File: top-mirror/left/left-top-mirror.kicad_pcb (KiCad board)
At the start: 2 copper layers, 137.8 x 95 mm, 30 parts

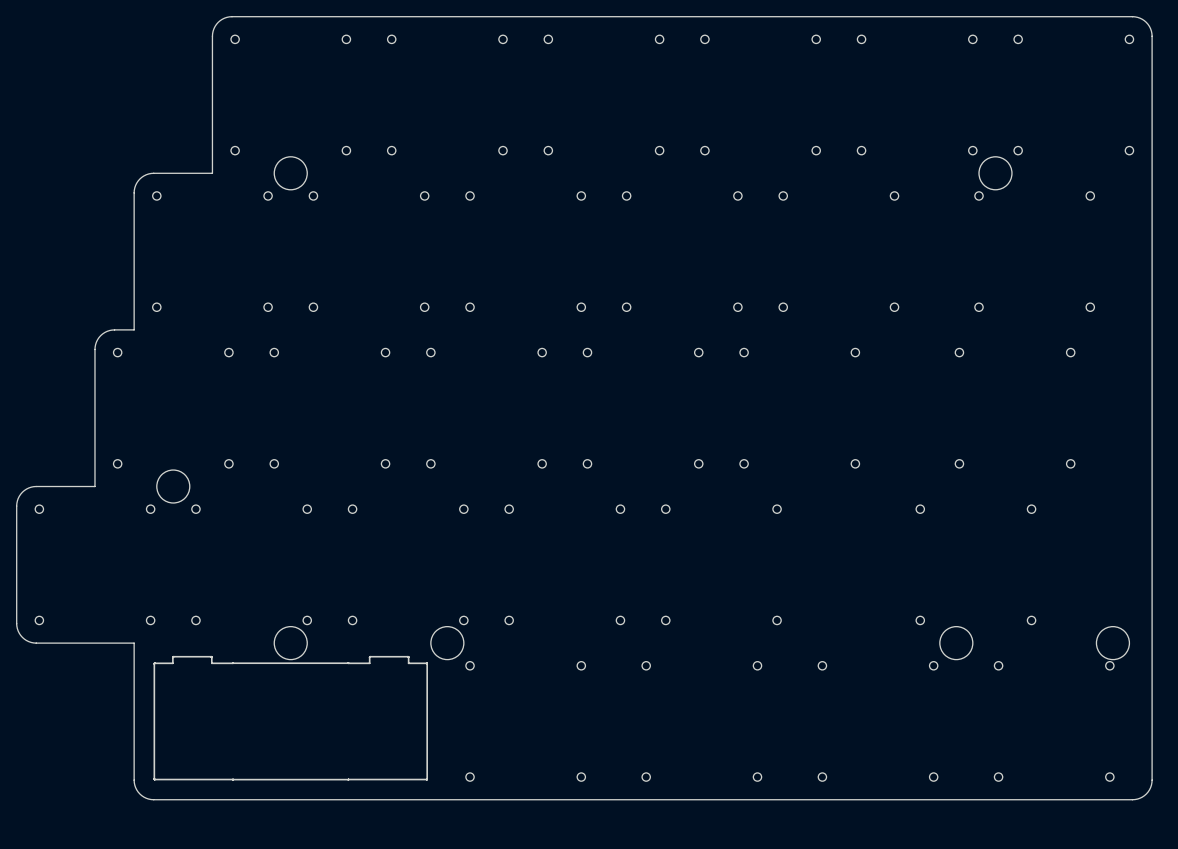
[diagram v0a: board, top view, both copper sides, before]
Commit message: rev1 release
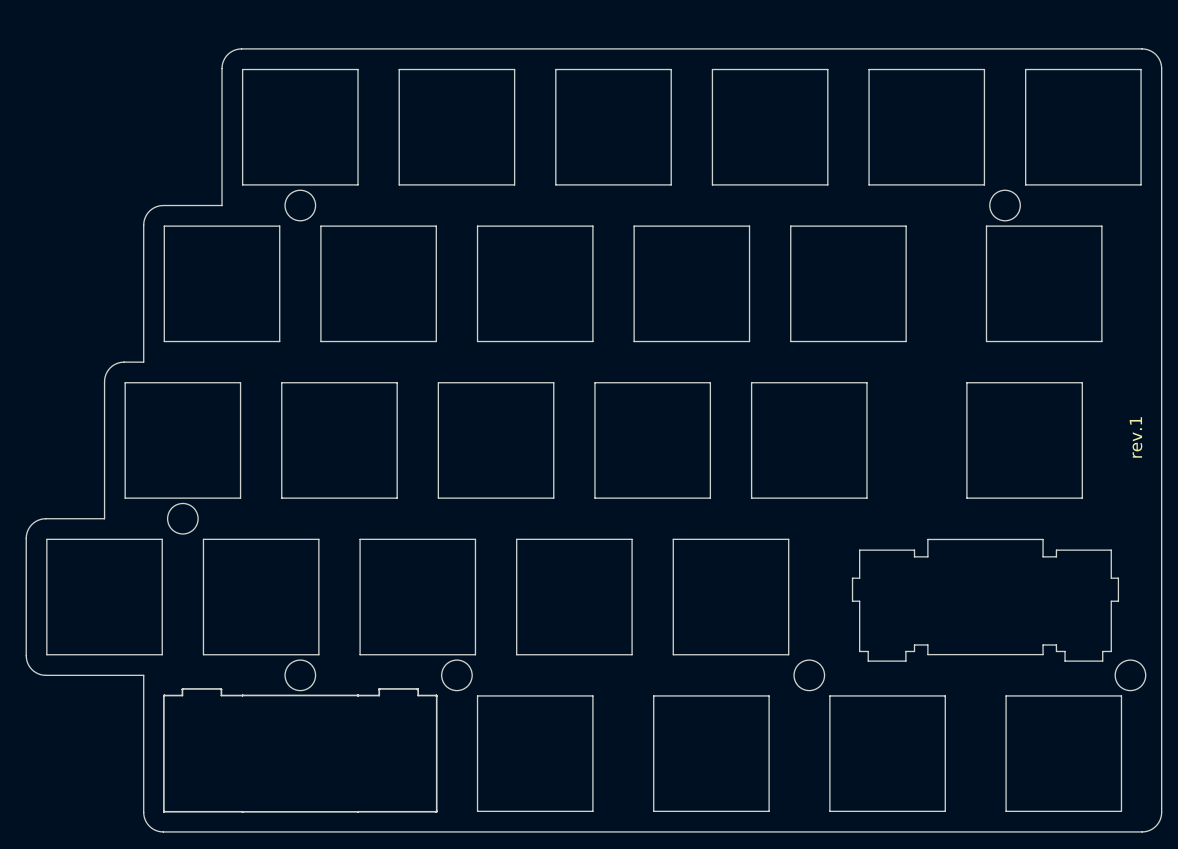
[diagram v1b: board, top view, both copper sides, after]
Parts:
- removed the MX_CUTOUT at (95.0, 47.5)
- removed the MX_CUTOUT at (90.2, 104.5)
- removed the MX_CUTOUT at (109.2, 104.5)
- removed the MX_CUTOUT at (128.2, 104.5)
- removed the MX_CUTOUT at (123.5, 123.5)
- removed the MX_CUTOUT at (144.9, 123.5)
- removed the MX_CUTOUT at (187.6, 123.5)
- removed the MX_CUTOUT at (166.2, 123.5)
- removed the MX_CUTOUT at (147.2, 104.5)
- removed the MX_CUTOUT at (137.8, 85.5)
- removed the MX_CUTOUT at (156.8, 85.5)
- removed the MX_CUTOUT at (114.0, 47.5)
- removed the MX_CUTOUT at (142.5, 66.5)
- removed the MX_CUTOUT at (161.5, 66.5)
- removed the MX_CUTOUT at (133.0, 47.5)
- removed the MX_CUTOUT at (152.0, 47.5)
- removed the MX_CUTOUT at (171.0, 47.5)
- removed the MX_CUTOUT at (190.0, 47.5)
- removed the MX_CUTOUT at (185.2, 66.5)
- removed the MX_CUTOUT at (182.9, 85.5)
- removed the MX_CUTOUT at (178.1, 104.5)
- removed the MX_CUTOUT at (85.5, 66.5)
- removed the MX_CUTOUT at (104.5, 66.5)
- removed the MX_CUTOUT at (123.5, 66.5)
- removed the MX_CUTOUT at (80.8, 85.5)
- removed the MX_CUTOUT at (71.2, 104.5)
- removed the MX_CUTOUT at (118.8, 85.5)
- removed the MX_CUTOUT at (99.8, 85.5)
- removed the REF** at (178.1, 104.5)
- added CHERRY: MX, lib:MX_PCB_CUTOUT, B.Cu at (179.3, 108.4)
- added MX_CUTOUT: VAL**, lib:MX_CUTOUT, B.Cu at (91.4, 108.4)
- added MX_CUTOUT: VAL**, lib:MX_CUTOUT, B.Cu at (96.2, 51.4)
- added MX_CUTOUT: VAL**, lib:MX_CUTOUT, B.Cu at (184.0, 89.4)
- added MX_CUTOUT: VAL**, lib:MX_CUTOUT, B.Cu at (129.4, 108.4)
- added MX_CUTOUT: VAL**, lib:MX_CUTOUT, B.Cu at (186.4, 70.4)
- added MX_CUTOUT: VAL**, lib:MX_CUTOUT, B.Cu at (157.9, 89.4)
- added MX_CUTOUT: VAL**, lib:MX_CUTOUT, B.Cu at (124.7, 127.4)
- added MX_CUTOUT: VAL**, lib:MX_CUTOUT, B.Cu at (188.8, 127.4)
- added MX_CUTOUT: VAL**, lib:MX_CUTOUT, B.Cu at (146.0, 127.4)
- added MX_CUTOUT: VAL**, lib:MX_CUTOUT, B.Cu at (143.7, 70.4)
- added MX_CUTOUT: VAL**, lib:MX_CUTOUT, B.Cu at (191.2, 51.4)
- added MX_CUTOUT: VAL**, lib:MX_CUTOUT, B.Cu at (167.4, 127.4)
- added MX_CUTOUT: VAL**, lib:MX_CUTOUT, B.Cu at (110.4, 108.4)
- added MX_CUTOUT: VAL**, lib:MX_CUTOUT, B.Cu at (148.4, 108.4)
- added MX_CUTOUT: VAL**, lib:MX_CUTOUT, B.Cu at (115.2, 51.4)
- added MX_CUTOUT: VAL**, lib:MX_CUTOUT, B.Cu at (86.7, 70.4)
- added MX_CUTOUT: VAL**, lib:MX_CUTOUT, B.Cu at (105.7, 70.4)
- added MX_CUTOUT: VAL**, lib:MX_CUTOUT, B.Cu at (72.4, 108.4)
- added MX_CUTOUT: VAL**, lib:MX_CUTOUT, B.Cu at (81.9, 89.4)
- added MX_CUTOUT: VAL**, lib:MX_CUTOUT, B.Cu at (124.7, 70.4)
- added MX_CUTOUT: VAL**, lib:MX_CUTOUT, B.Cu at (172.2, 51.4)
- added MX_CUTOUT: VAL**, lib:MX_CUTOUT, B.Cu at (138.9, 89.4)
- added MX_CUTOUT: VAL**, lib:MX_CUTOUT, B.Cu at (100.9, 89.4)
- added MX_CUTOUT: VAL**, lib:MX_CUTOUT, B.Cu at (153.2, 51.4)
- added MX_CUTOUT: VAL**, lib:MX_CUTOUT, B.Cu at (119.9, 89.4)
- added MX_CUTOUT: VAL**, lib:MX_CUTOUT, B.Cu at (162.7, 70.4)
- added MX_CUTOUT: VAL**, lib:MX_CUTOUT, B.Cu at (134.2, 51.4)
- added REF**: MountingHole_3.7mm, MountingHole:MountingHole_3.7mm, B.Cu at (181.7, 60.9)
- added REF**: MountingHole_3.7mm, MountingHole:MountingHole_3.7mm, B.Cu at (115.2, 117.9)
- added REF**: MountingHole_3.7mm, MountingHole:MountingHole_3.7mm, B.Cu at (198.9, 117.6)
- added REF**: MountingHole_3.7mm, MountingHole:MountingHole_3.7mm, B.Cu at (157.9, 117.9)
- added REF**: MountingHole_3.7mm, MountingHole:MountingHole_3.7mm, B.Cu at (96.2, 117.9)
- added REF**: MountingHole_3.7mm, MountingHole:MountingHole_3.7mm, B.Cu at (96.2, 60.9)
- added REF**: MountingHole_3.7mm, MountingHole:MountingHole_3.7mm, B.Cu at (81.9, 98.9)
- moved REF** 4.08 mm to (96.2, 127.4)
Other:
- outline, holes or cut-outs redrawn
- board text added: "rev.1"
